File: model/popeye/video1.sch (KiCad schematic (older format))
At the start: 39 parts, among them U3R1 74LS283, U3S1 74LS283, U3T1 74LS283, U5 74LS174, U6 74LS174, U7 74LS174

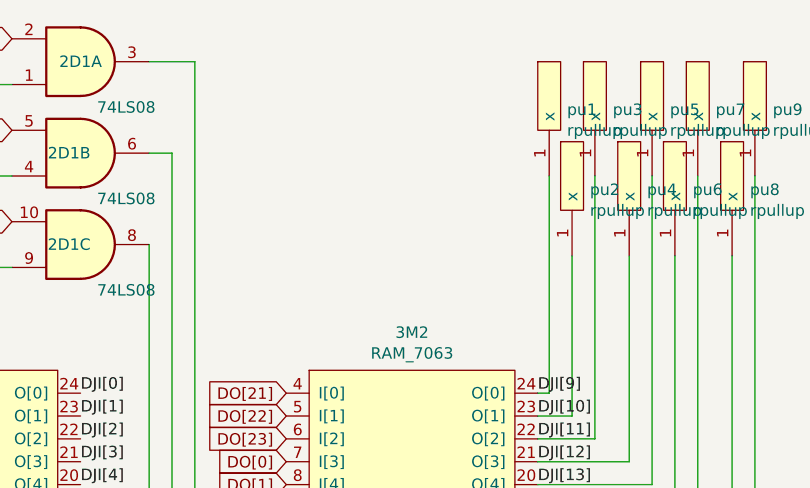
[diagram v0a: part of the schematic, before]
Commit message: wip
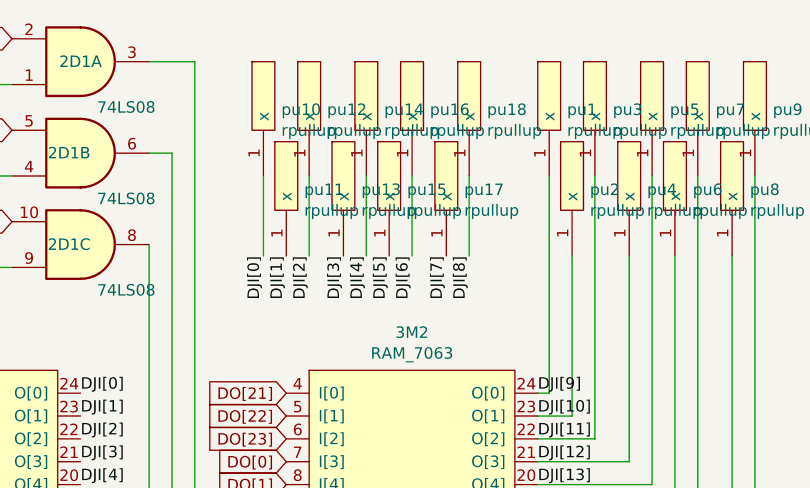
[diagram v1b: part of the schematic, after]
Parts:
- added pu10, pu11, pu12, pu13, pu14, pu15, pu16, pu17, pu18: rpullup, symbol arcade:rpullup
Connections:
- net DJI[0]: now also pu10.1 (x)
- net DJI[1]: now also pu11.1 (x)
- net DJI[2]: now also pu12.1 (x)
- net DJI[3]: now also pu13.1 (x)
- net DJI[4]: now also pu14.1 (x)
- net DJI[5]: now also pu15.1 (x)
- net DJI[6]: now also pu16.1 (x)
- net DJI[7]: now also pu17.1 (x)
- net DJI[8]: now also pu18.1 (x)
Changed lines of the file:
@@
 Wire Wire Line
 	4400 9350 4450 9350
+$Comp
+L arcade:rpullup pu10
+U 1 1 5DB34EC5
+P 15400 2500
+F 0 "pu10" H 15478 2790 50  0000 L CNN
+F 1 "rpullup" H 15478 2699 50  0000 L CNN
+F 2 "" H 15200 2500 50  0001 C CNN
+F 3 "" H 15200 2500 50  0001 C CNN
+	1    15400 2500
+	1    0    0    -1
+$EndComp
+$Comp
+L arcade:rpullup pu11
+U 1 1 5DB34ECC
+P 15500 2850
+F 0 "pu11" H 15578 3140 50  0000 L CNN
+F 1 "rpullup" H 15578 3049 50  0000 L CNN
+F 2 "" H 15300 2850 50  0001 C CNN
+F 3 "" H 15300 2850 50  0001 C CNN
+	1    15500 2850
+	1    0    0    -1
+$EndComp
+$Comp
+L arcade:rpullup pu12
+U 1 1 5DB34ED3
+P 15600 2500
+F 0 "pu12" H 15678 2790 50  0000 L CNN
+F 1 "rpullup" H 15678 2699 50  0000 L CNN
+F 2 "" H 15400 2500 50  0001 C CNN
+F 3 "" H 15400 2500 50  0001 C CNN
+	1    15600 2500
+	1    0    0    -1
+$EndComp
+$Comp
+L arcade:rpullup pu13
+U 1 1 5DB34EDA
+P 15750 2850
+F 0 "pu13" H 15828 3140 50  0000 L CNN
+F 1 "rpullup" H 15828 3049 50  0000 L CNN
+F 2 "" H 15550 2850 50  0001 C CNN
+F 3 "" H 15550 2850 50  0001 C CNN
+	1    15750 2850
+	1    0    0    -1
+$EndComp
+$Comp
+L arcade:rpullup pu14
+U 1 1 5DB34EE1
+P 15850 2500
+F 0 "pu14" H 15928 2790 50  0000 L CNN
+F 1 "rpullup" H 15928 2699 50  0000 L CNN
+F 2 "" H 15650 2500 50  0001 C CNN
+F 3 "" H 15650 2500 50  0001 C CNN
+	1    15850 2500
+	1    0    0    -1
+$EndComp
+$Comp
+L arcade:rpullup pu15
+U 1 1 5DB34EE8
+P 15950 2850
+F 0 "pu15" H 16028 3140 50  0000 L CNN
+F 1 "rpullup" H 16028 3049 50  0000 L CNN
+F 2 "" H 15750 2850 50  0001 C CNN
+F 3 "" H 15750 2850 50  0001 C CNN
+	1    15950 2850
+	1    0    0    -1
+$EndComp
+$Comp
+L arcade:rpullup pu16
+U 1 1 5DB34EEF
+P 16050 2500
+F 0 "pu16" H 16128 2790 50  0000 L CNN
+F 1 "rpullup" H 16128 2699 50  0000 L CNN
+F 2 "" H 15850 2500 50  0001 C CNN
+F 3 "" H 15850 2500 50  0001 C CNN
+	1    16050 2500
+	1    0    0    -1
+$EndComp
+$Comp
+L arcade:rpullup pu17
+U 1 1 5DB34EF6
+P 16200 2850
+F 0 "pu17" H 16278 3140 50  0000 L CNN
+F 1 "rpullup" H 16278 3049 50  0000 L CNN
+F 2 "" H 16000 2850 50  0001 C CNN
+F 3 "" H 16000 2850 50  0001 C CNN
+	1    16200 2850
+	1    0    0    -1
+$EndComp
+$Comp
+L arcade:rpullup pu18
+U 1 1 5DB34EFD
+P 16300 2500
+F 0 "pu18" H 16378 2790 50  0000 L CNN
+F 1 "rpullup" H 16378 2699 50  0000 L CNN
+F 2 "" H 16100 2500 50  0001 C CNN
+F 3 "" H 16100 2500 50  0001 C CNN
+	1    16300 2500
+	1    0    0    -1
+$EndComp
+Text Label 15400 2850 3    50   ~ 0
+DJI[0]
+Text Label 15500 2850 3    50   ~ 0
+DJI[1]
+Text Label 15600 2850 3    50   ~ 0
+DJI[2]
+Wire Wire Line
+	15600 2850 15600 2500
+Wire Wire Line
+	15400 2500 15400 2850
+Wire Wire Line
+	15850 2500 15850 2850
+Text Label 15750 2850 3    50   ~ 0
+DJI[3]
+Text Label 15850 2850 3    50   ~ 0
+DJI[4]
+Text Label 15950 2850 3    50   ~ 0
+DJI[5]
+Text Label 16050 2850 3    50   ~ 0
+DJI[6]
+Text Label 16200 2850 3    50   ~ 0
+DJI[7]
+Text Label 16300 2850 3    50   ~ 0
+DJI[8]
+Wire Wire Line
+	16300 2850 16300 2500
+Wire Wire Line
+	16050 2850 16050 2500
 $EndSCHEMATC
